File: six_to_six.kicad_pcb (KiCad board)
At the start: 2 copper layers, 190.5 x 88.9 mm, 76 parts, among them J1 pads for coax, J2 pads for coax, J3 pads for coax, J4 pads for coax, J5 pads for coax, J6 pads for coax, J7 BNC, J8 Relay control, K1 RY-12W-K, K2 RY-12W-K, K3 RY-12W-K, K4 RY-12W-K, K5 RY-12W-K, K6 RY-12W-K, Q1 MMBT3904, Q2 MMBT3904, Q3 MMBT3904, Q4 MMBT3904, Q5 MMBT3904, Q6 MMBT3904

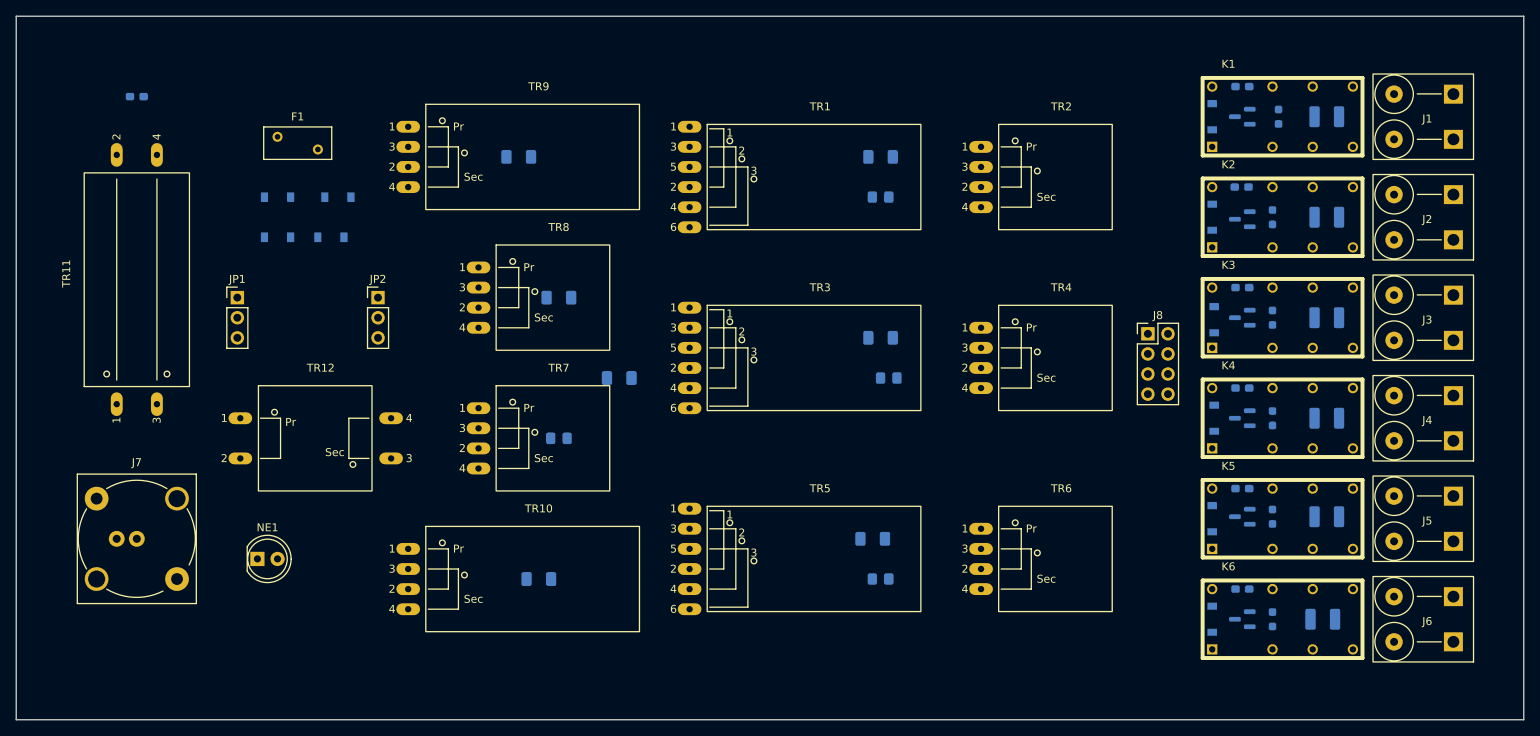
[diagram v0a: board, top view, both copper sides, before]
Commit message: pcb routed and made gerbers
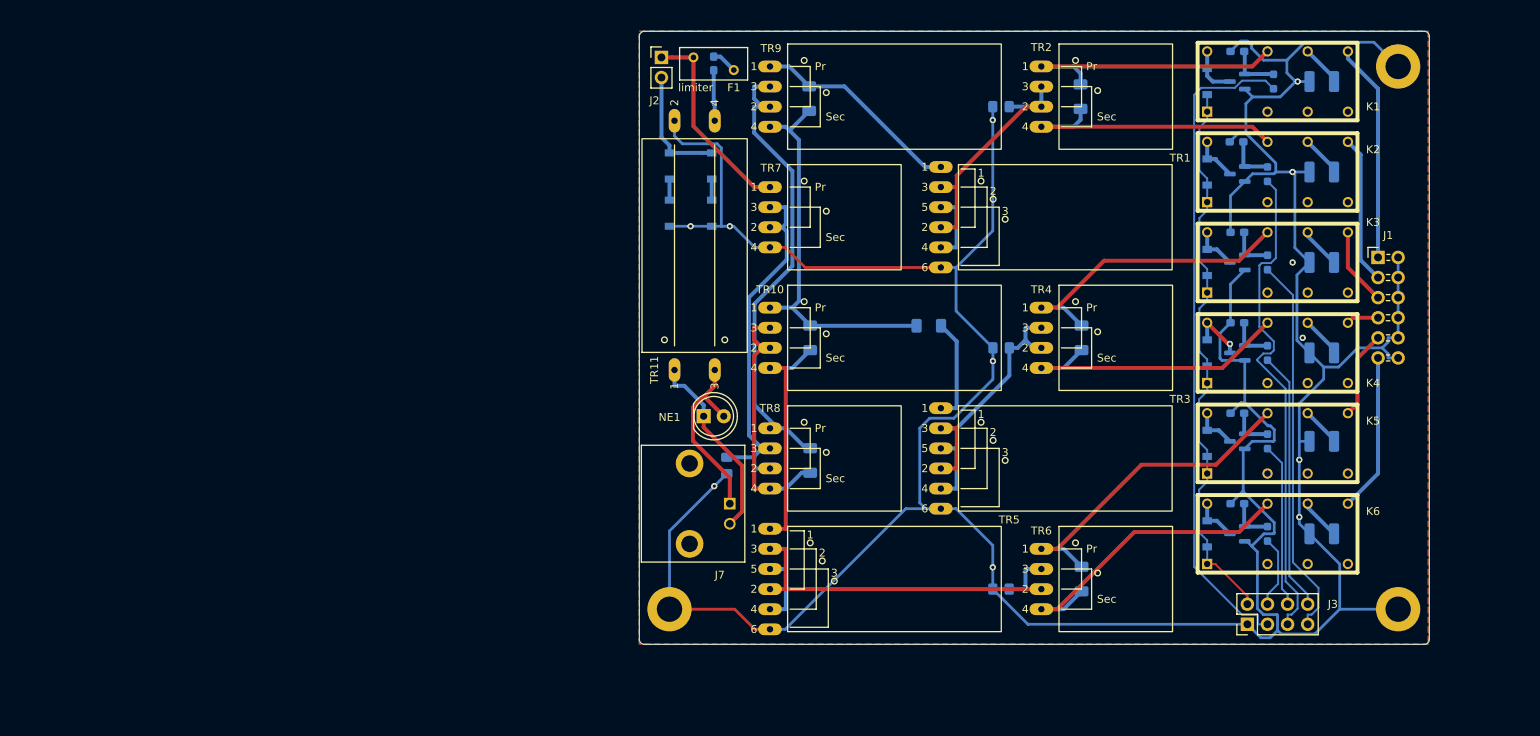
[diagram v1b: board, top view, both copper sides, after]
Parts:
- removed J4, J5, J6: pads for coax, Components:Coax_pad
- removed J8: Relay control, Connector_PinHeader_2.54mm:PinHeader_2x04_P2.54mm_Vertical
- removed JP1, JP2: 50/75 ohm, Connector_PinHeader_2.54mm:PinHeader_1x03_P2.54mm_Vertical
- removed TR12: BN-73-transformer, Components:BN-73-202-1-1
- added H1: M3, MountingHole:MountingHole_3.2mm_M3_DIN965_Pad, F.Cu at (646.4, 232.4)
- added H2: M3, MountingHole:MountingHole_3.2mm_M3_DIN965_Pad, F.Cu at (738.5, 232.4)
- added H3: M3, MountingHole:MountingHole_3.2mm_M3_DIN965_Pad, F.Cu at (738.5, 163.8)
- J1: value pads for coax -> RF Conn; footprint Components:Coax_pad -> Components:PinHeader_2x06_P2.54mm_Horizontal
- J2: value pads for coax -> limiter; footprint Components:Coax_pad -> Connector_PinHeader_2.54mm:PinHeader_1x02_P2.54mm_Vertical
- J3: value pads for coax -> Relay control; footprint Components:Coax_pad -> Connector_PinHeader_2.54mm:PinHeader_2x04_P2.54mm_Vertical
- J7: footprint Components:BNC_vertical -> Components:BNC_horizontal
- moved J2 102.7 mm to (645.4, 162.7), turned to 0 degrees
- moved C10 73.0 mm to (652.0, 163.4), turned to 90 degrees
- moved TR11 70.6 mm to (647.1, 202.2)
- moved J7 70.0 mm to (649.0, 219.1), turned to 90 degrees
- moved NE1 59.2 mm to (650.7, 208.0)
- moved F1 58.3 mm to (654.6, 164.3), turned to 180 degrees
- moved D10 55.6 mm to (651.8, 176.4), turned to -90 degrees
- moved TR10 54.9 mm to (659.1, 194.3)
- moved D7 54.9 mm to (651.8, 182.4), turned to -90 degrees
- moved TR9 46.4 mm to (659.1, 163.8)
- moved TR7 46.2 mm to (659.1, 179.1)
- moved R18 45.9 mm to (664.2, 198.1), turned to -90 degrees
- moved J3 44.3 mm to (719.5, 234.3), turned to 90 degrees
- moved D9 42.9 mm to (646.4, 182.4), turned to 90 degrees
- moved D8 42.1 mm to (646.4, 176.4), turned to 90 degrees
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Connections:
- D10 pad 1: Net-(D8-Pad2) -> Net-(D10-Pad1)
- D8 pad 2: Net-(D8-Pad2) -> Net-(D10-Pad1)
- F1 pad 2: Net-(D8-Pad2) -> /One to Six splitter/3-Way Splitter/RF-in
- J1 pad 1: GND -> /One to Six splitter/Connectors/RF-1
- J1 pad 2: Net-(K1-Pad9) -> GND
- J2 pad 1: GND -> /One to Six splitter/3-Way Splitter/RF-in
- J2 pad 2: Net-(K2-Pad9) -> Net-(D10-Pad1)
- J3 pad 2: Net-(K3-Pad9) -> +12V
- K1 pad 9: Net-(K1-Pad9) -> /One to Six splitter/Connectors/RF-1
- K2 pad 9: Net-(K2-Pad9) -> /One to Six splitter/Connectors/RF-2
- K3 pad 9: Net-(K3-Pad9) -> /One to Six splitter/Connectors/RF-3
- K4 pad 9: Net-(K4-Pad9) -> /One to Six splitter/Connectors/RF-4
- K5 pad 9: Net-(J5-Pad2) -> /One to Six splitter/Connectors/RF-5
- K6 pad 9: Net-(K6-Pad9) -> /One to Six splitter/Connectors/RF-6
- TR11 pad 1: Net-(J7-Pad1) -> Net-(J7-Pad2)
- TR11 pad 2: Net-(C10-Pad1) -> GND
- TR11 pad 3: Net-(J7-Pad2) -> Net-(J7-Pad1)
- TR11 pad 4: GND -> Net-(C10-Pad1)
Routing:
- net GND: track 0.00 -> 469.5 mm, vias 0 -> 12
- net /One to Six splitter/Connectors/Relay-1: track 0.00 -> 83.8 mm
- net +12V: track 0.00 -> 71.3 mm
- net /One to Six splitter/Connectors/Relay-2: track 0.00 -> 63.1 mm
- net Net-(R16-Pad1): track 0.00 -> 58.9 mm
- net Net-(C9-Pad1): track 0.00 -> 50.0 mm
- net Net-(R17-Pad2): track 0.00 -> 48.9 mm
- net /One to Six splitter/Connectors/Relay-3: track 0.00 -> 48.3 mm
- net Net-(C11-Pad1): track 0.00 -> 46.5 mm
- net /One to Six splitter/2-Way Splitter3/RF-out-1: track 0.00 -> 41.7 mm
- net /One to Six splitter/2-Way Splitter3/RF-out-2: track 0.00 -> 40.1 mm
- net /One to Six splitter/2-Way Splitter2/RF-out-1: track 0.00 -> 38.5 mm
- net /One to Six splitter/2-Way Splitter2/RF-out-2: track 0.00 -> 37.0 mm
- net /One to Six splitter/2-Way Splitter1/RF-out-2: track 0.00 -> 36.1 mm
- net /One to Six splitter/2-Way Splitter1/RF-out-1: track 0.00 -> 36.1 mm
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- added copper zone on B.Cu, net GND
- added copper zone on F.Cu, net GND
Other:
- board size 190.5 x 88.9 mm -> 99.8 x 77.5 mm
